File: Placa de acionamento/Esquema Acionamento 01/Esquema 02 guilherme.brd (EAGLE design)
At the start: 66 x 57.2 mm, 22 parts, among them Q1 IRF540, Q2 IRF540, Q3 IRF540

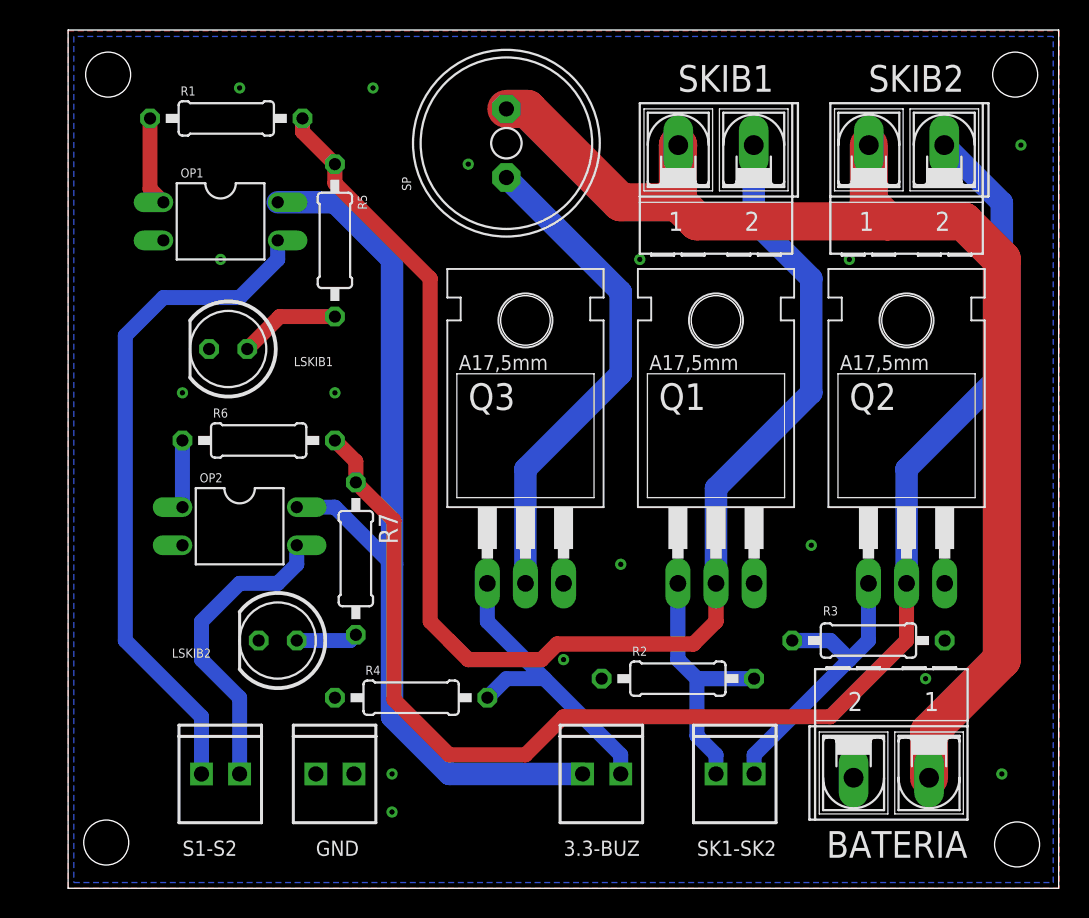
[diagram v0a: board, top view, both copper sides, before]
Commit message: Placa de acionamento
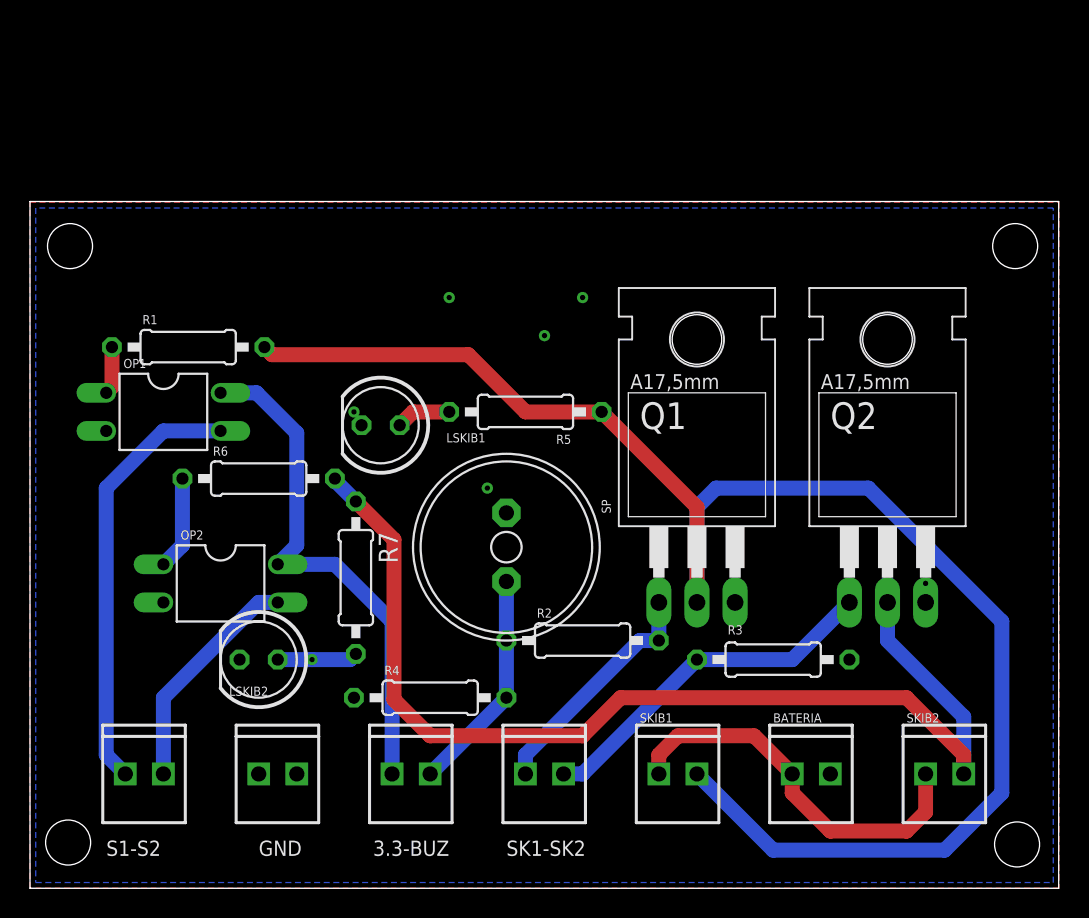
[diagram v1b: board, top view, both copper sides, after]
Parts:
- removed Q3: IRF540, transistor-fet:TO220
- BATERIA, SKIB1, SKIB2: device con-ptr500:AK500/2-H -> SparkFun-Connectors:1X02_2.54_SCREWTERM
- moved SKIB1 42.1 mm to (39.4, 7.62)
- moved SKIB2 41.9 mm to (57.1, 7.62)
- moved SP 26.9 mm to (29.2, 22.7), turned to 270 degrees
- moved R5 17.1 mm to (30.5, 31.8), turned to 180 degrees
- moved R1 15.5 mm to (8.00, 36.1)
- moved OP1 13.3 mm to (6.35, 31.8)
- moved 3.3-BUZ 12.7 mm to (21.6, 7.62)
- moved SK1-SK2 12.7 mm to (30.5, 7.62)
- moved LSKIB1 11.4 mm to (20.8, 30.9)
- moved R2 6.84 mm to (34.3, 16.5)
- moved BATERIA 6.61 mm to (48.3, 7.62), turned to 0 degrees
- moved R3 6.48 mm to (47.0, 15.2)
- moved S1-S2 5.08 mm to (3.81, 7.62)
- moved OP2 4.02 mm to (10.2, 20.3)
- moved GND 3.81 mm to (12.7, 7.62)
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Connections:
- removed net N$2: Q3.2, SP.-
- net BUZZER: now also SP.+; no longer Q3.1
- net GND: now also BATERIA.P1, SP.-; no longer BATERIA.2, Q3.3
- net SKIB1_CONECTOR: now also SKIB1.P1; no longer SKIB1.2
- net SKIB2_CONECTOR: now also SKIB2.P1; no longer SKIB2.2
- net VCC: now also BATERIA.P2, SKIB1.P2, SKIB2.P2; no longer BATERIA.1, SKIB1.1, SKIB2.1, SP.+
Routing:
- net VCC: track 83.2 -> 26.1 mm
- net N$2: track 32.8 -> 0.00 mm
- net 3.3V: track 61.9 -> 34.8 mm
- net SKIB2_CONECTOR: track 95.0 -> 74.0 mm
- net SINAL_SKIB1: track 44.8 -> 28.8 mm
- net SKIB1_CONECTOR: track 94.2 -> 105.9 mm
- net BUZZER: track 20.7 -> 14.9 mm
- net SINAL_SKIB2: track 20.4 -> 15.3 mm
- net SKIB2: track 20.2 -> 23.8 mm
- net N$3: track 6.74 -> 3.67 mm
- net N$4: track 5.96 -> 3.21 mm
- net N$5: track 4.45 -> 6.24 mm
- net SKIB1: track 17.6 -> 15.9 mm
- net N$1: track 4.09 -> 5.36 mm, vias 0 -> 1
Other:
- board size 66 x 57.2 mm -> 68.6 x 45.8 mm
